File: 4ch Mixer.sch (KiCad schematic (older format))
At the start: 42 parts, among them J1 JACK_2P, J2 JACK_2P, J3 JACK_2P, J4 JACK_2P, J5 JACK_2P, J6 JACK_2P, P1 CONN_02X08, U1 TL074, U2 TL072

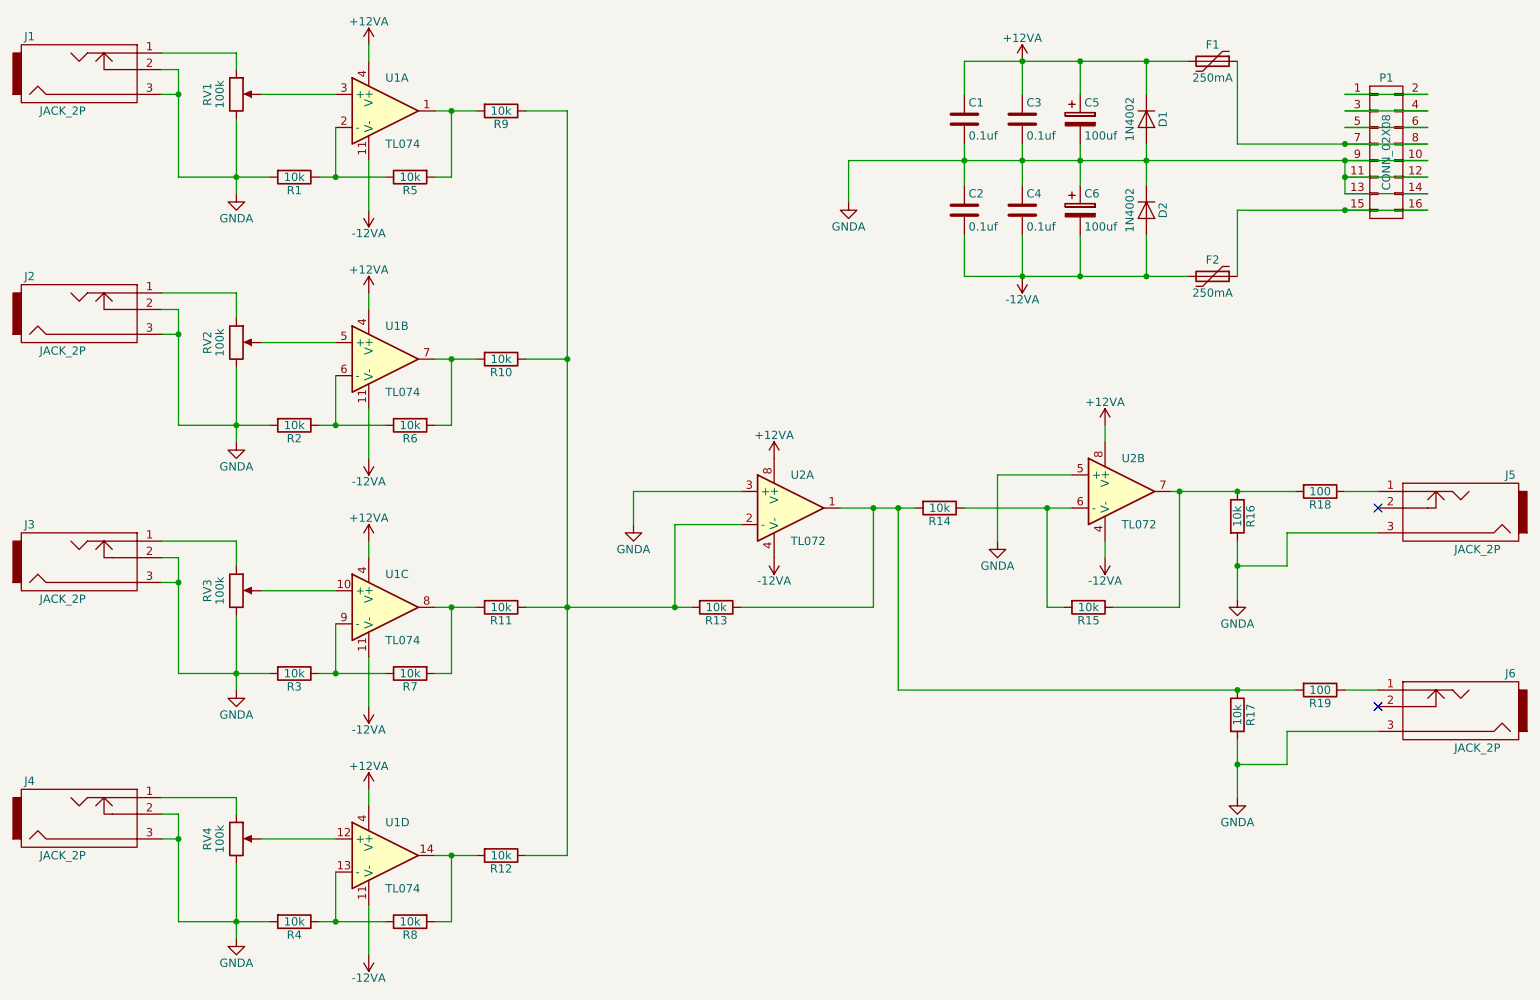
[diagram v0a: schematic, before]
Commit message: Continued work on PCB and Schematic
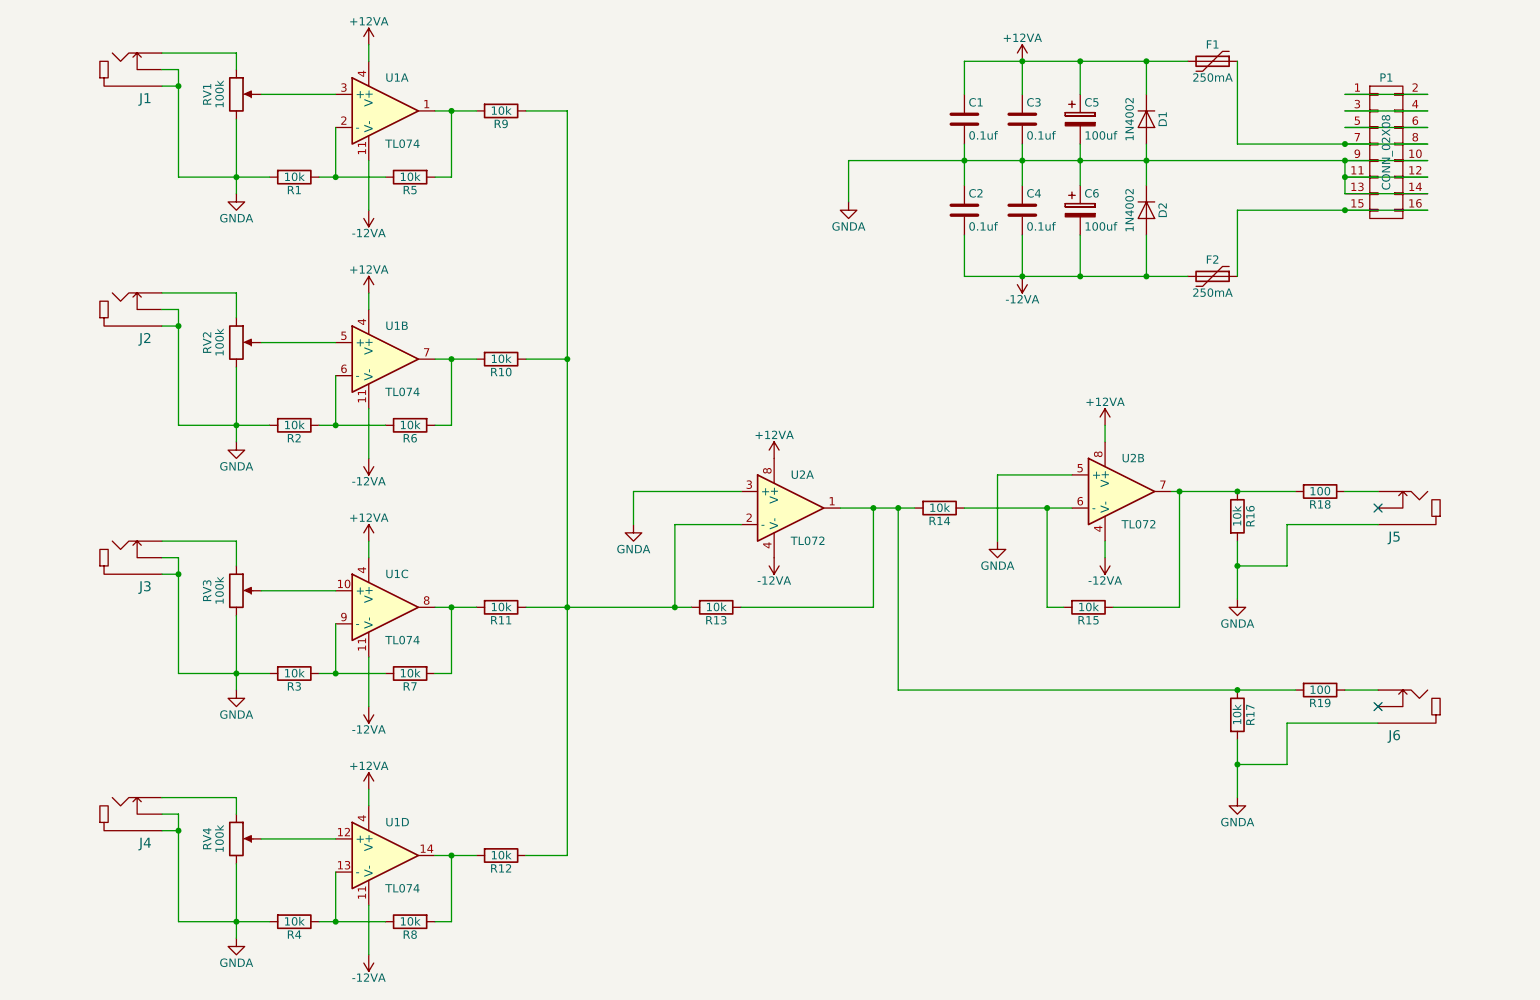
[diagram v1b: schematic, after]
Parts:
- removed J1, J2, J3, J4, J5, J6: JACK_2P, Connectors:JACK_ALIM, symbol JACK_2P
- added J1, J2, J3, J4, J5, J6: 3.5mm_Mono_Jack_With_Switch, _NTSFootprints:3.5mm_Mono_Vertical_QuingPu_WQP-PJ301M-12, symbol 3.5mm_Mono_Jack_With_Switch
- C1, C2, C3, C4: footprint Capacitors_THT:C_Rect_L11.0mm_W3.4mm_P10.00mm_MKT -> Capacitors_THT:C_Axial_L5.1mm_D3.1mm_P10.00mm_Horizontal
- C5, C6: footprint Capacitors_THT:CP_Radial_D10.0mm_P7.50mm -> Capacitors_THT:CP_Radial_D8.0mm_P5.00mm
- D1, D2: footprint Diodes_THT:D_DO-15_P12.70mm_Horizontal -> Diodes_THT:D_DO-35_SOD27_P2.54mm_Vertical_AnodeUp
- R1, R10, R11, R12, R13, R14, R15, R16, R17, R18, R19, R2, R3, R4, R5, R6, R7, R8, R9: footprint Resistors_THT:R_Axial_DIN0309_L9.0mm_D3.2mm_P12.70mm_Horizontal -> Resistors_THT:R_Axial_DIN0207_L6.3mm_D2.5mm_P2.54mm_Vertical
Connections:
- net GNDA: now also J1.1, J1.2, J2.1, J2.2, J3.1, J3.2, J4.1, J4.2, J5.1, J6.1
- net at RV1.1: now also J1.3
- net at RV2.1: now also J2.3
- net at RV3.1: now also J3.3
- net at RV4.1: now also J4.3
- net at R18.1: now also J5.3
- net at R19.1: now also J6.3
